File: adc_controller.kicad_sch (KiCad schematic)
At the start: 7 parts, among them J3 Conn_01x06

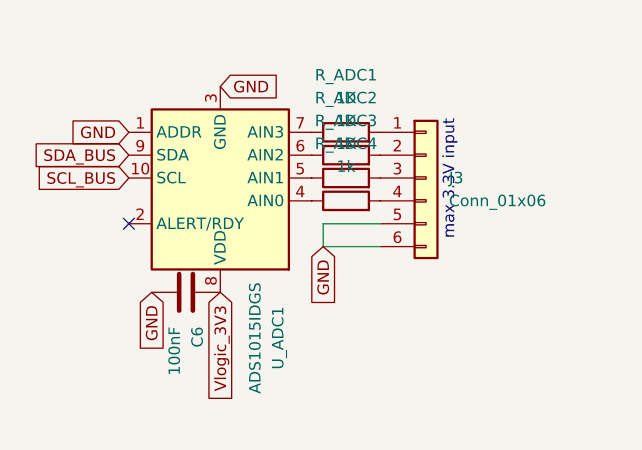
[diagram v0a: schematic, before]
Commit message: Add files via upload
v1.2 : complete schematics with added footprints, PCB layout remaining
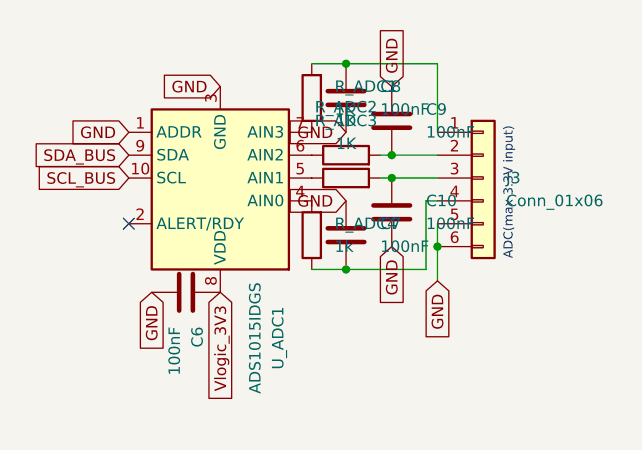
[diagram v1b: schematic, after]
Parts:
- added C10, C7, C8, C9: 100nF, Capacitor_SMD:C_0805_2012Metric, symbol Device:C
- J3: footprint (none) -> Connector_PinSocket_2.54mm:PinSocket_1x06_P2.54mm_Vertical
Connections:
- net GND: now also C10.2, C7.1, C8.2, C9.1
- net at J3.2 (Pin_2), R_ADC2.2: now also C9.2
- net at U_ADC1.4 (AIN0): now also R_ADC4.2; no longer R_ADC4.1
- net at J3.1 (Pin_1), R_ADC1.2: now also C8.1
- net at J3.3 (Pin_3), R_ADC3.2: now also C10.1
- net at J3.4 (Pin_4): now also R_ADC4.1, C7.2; no longer R_ADC4.2
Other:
- note added: "ADC(max 3.3V input)"
- note removed: "max 3.3V input"
- moved on the sheet: J3, R_ADC1, R_ADC4

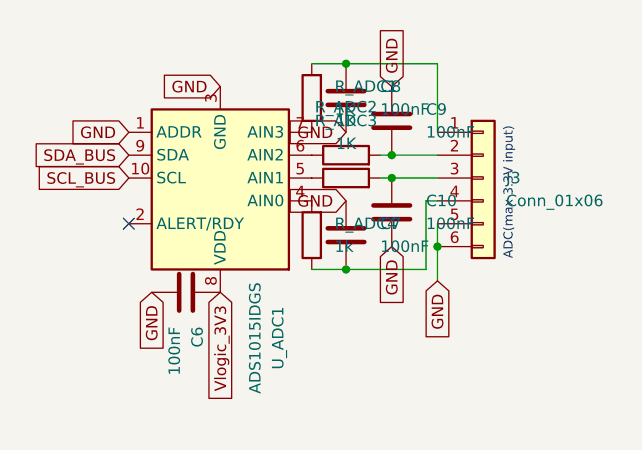
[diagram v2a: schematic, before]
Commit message: Add files via upload
V5 : complete finish for v1, directly to-the-fab design.
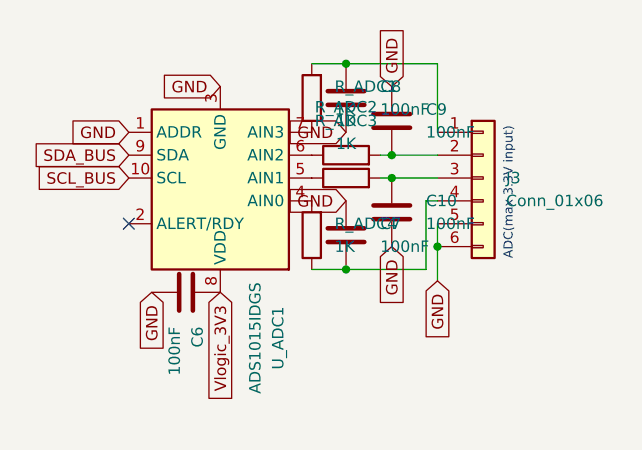
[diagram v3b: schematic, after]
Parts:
- C10, C6, C7, C8, C9: LCSC (none) -> C49678
- J3: LCSC (none) -> C40877
- R_ADC1, R_ADC2, R_ADC3: LCSC (none) -> C17513
- R_ADC4: value 1k -> 1K; LCSC (none) -> C17513
- U_ADC1: LCSC (none) -> C16581
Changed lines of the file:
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@@
+			)
+		)
+		(property "LCSC" "C17513"
+			(at 242.57 123.19 90)
+			(effects
+				(font
+					(size 1.27 1.27)
+				)
+				(hide yes)
 			)
 		)
@@
 			)
 		)
+		(property "LCSC" "C16581"
+			(at 228.6 125.73 90)
+			(effects
+				(font
+					(size 1.27 1.27)
+				)
+				(hide yes)
+			)
+		)
 		(pin "1"
 		)
@@
 			)
 		)
+		(property "LCSC" "C49678"
+			(at 242.57 116.84 0)
+			(effects
+				(font
+					(size 1.27 1.27)
+				)
+				(hide yes)
+			)
+		)
 		(pin "1"
 		)
@@
 			)
 		)
+		(property "LCSC" "C40877"
+			(at 257.81 125.73 0)
+			(effects
+				(font
+					(size 1.27 1.27)
+				)
+				(hide yes)
+			)
+		)
 		(pin "2"
 		)
@@
 			)
 		)
+		(property "LCSC" "C49678"
+			(at 247.65 119.38 0)
+			(effects
+				(font
+					(size 1.27 1.27)
+				)
+				(hide yes)
+			)
+		)
 		(pin "1"
 		)
@@
 			)
 		)
+		(property "LCSC" "C49678"
+			(at 242.57 132.08 0)
+			(effects
+				(font
+					(size 1.27 1.27)
+				)
+				(hide yes)
+			)
+		)
 		(pin "2"
 		)
@@
 			)
 		)
+		(property "LCSC" "C17513"
+			(at 242.57 125.73 90)
+			(effects
+				(font
+					(size 1.27 1.27)
+				)
+				(hide yes)
+			)
+		)
 		(pin "1"
 		)
@@
 			)
 		)
+		(property "LCSC" "C17513"
+			(at 238.76 116.84 0)
+			(effects
+				(font
+					(size 1.27 1.27)
+				)
+				(hide yes)
+			)
+		)
 		(pin "1"
 		)
@@
 			)
 		)
+		(property "LCSC" "C49678"
+			(at 247.65 129.54 0)
+			(effects
+				(font
+					(size 1.27 1.27)
+				)
+				(hide yes)
+			)
+		)
 		(pin "2"
 		)
@@
 			)
 		)
+		(property "LCSC" "C49678"
+			(at 224.79 138.43 0)
+			(effects
+				(font
+					(size 1.27 1.27)
+				)
+				(hide yes)
+			)
+		)
 		(pin "2"
 		)
@@
 			)
 		)
-		(property "Value" "1k"
+		(property "Value" "1K"
 			(at 241.3 133.3499 0)
 			(effects
@@
 			(at 238.76 132.08 0)
 			(effects
+				(font
+					(size 1.27 1.27)
+				)
+				(hide yes)
+			)
+		)
+		(property "LCSC" "C17513"
+			(at 238.76 132.08 0)
+			(effects
